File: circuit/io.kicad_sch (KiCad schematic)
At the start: 16 parts, among them J1 Micro_SD_Card, J2 Conn_01x22, J2 VGA, J9 SWD programmer, SW1 Reset, U1 Pico, U10 TXB0104D, U4 TXS0108EPW, U7 74LS393

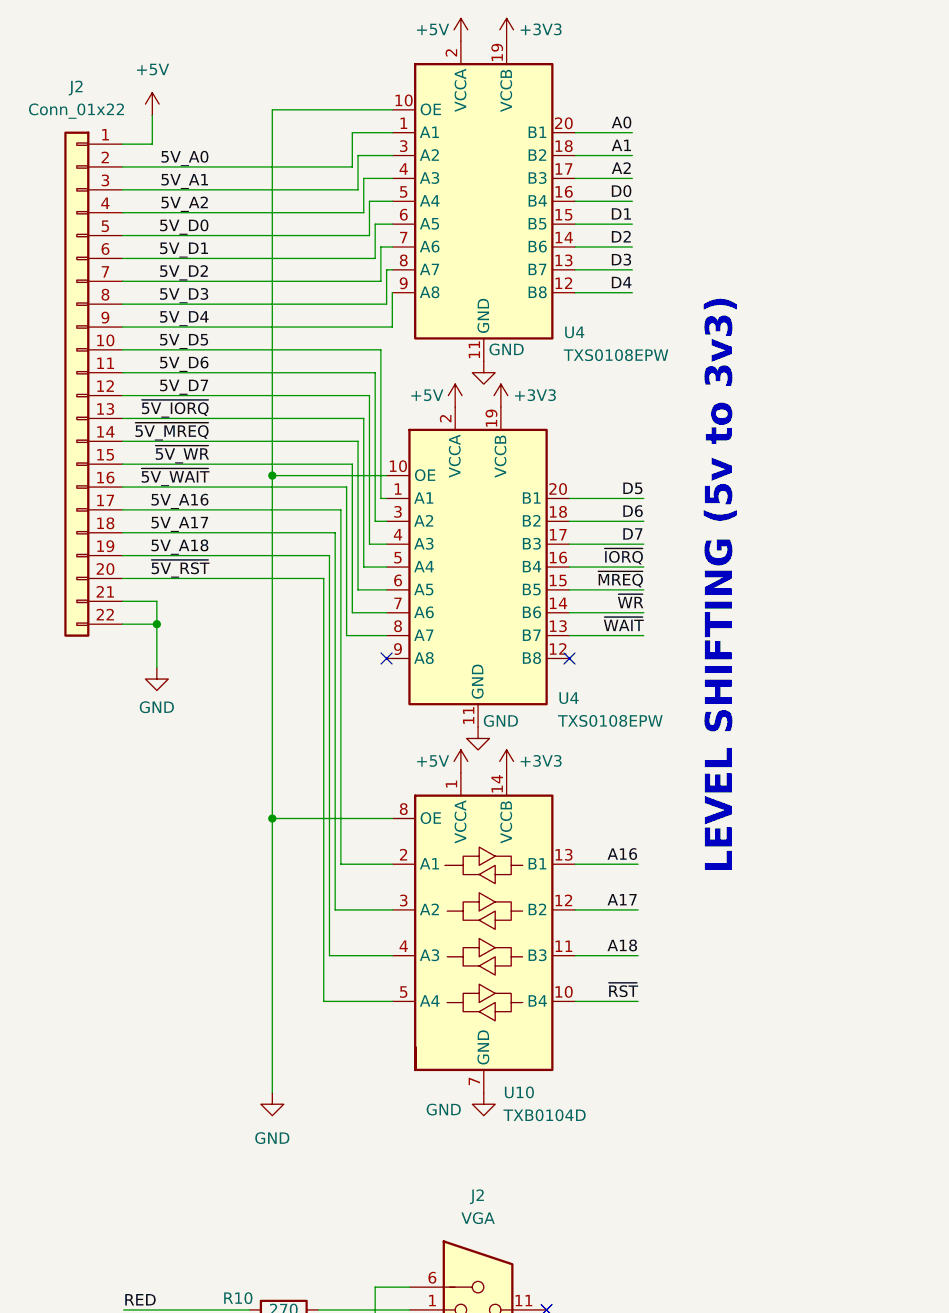
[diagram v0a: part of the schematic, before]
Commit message: .
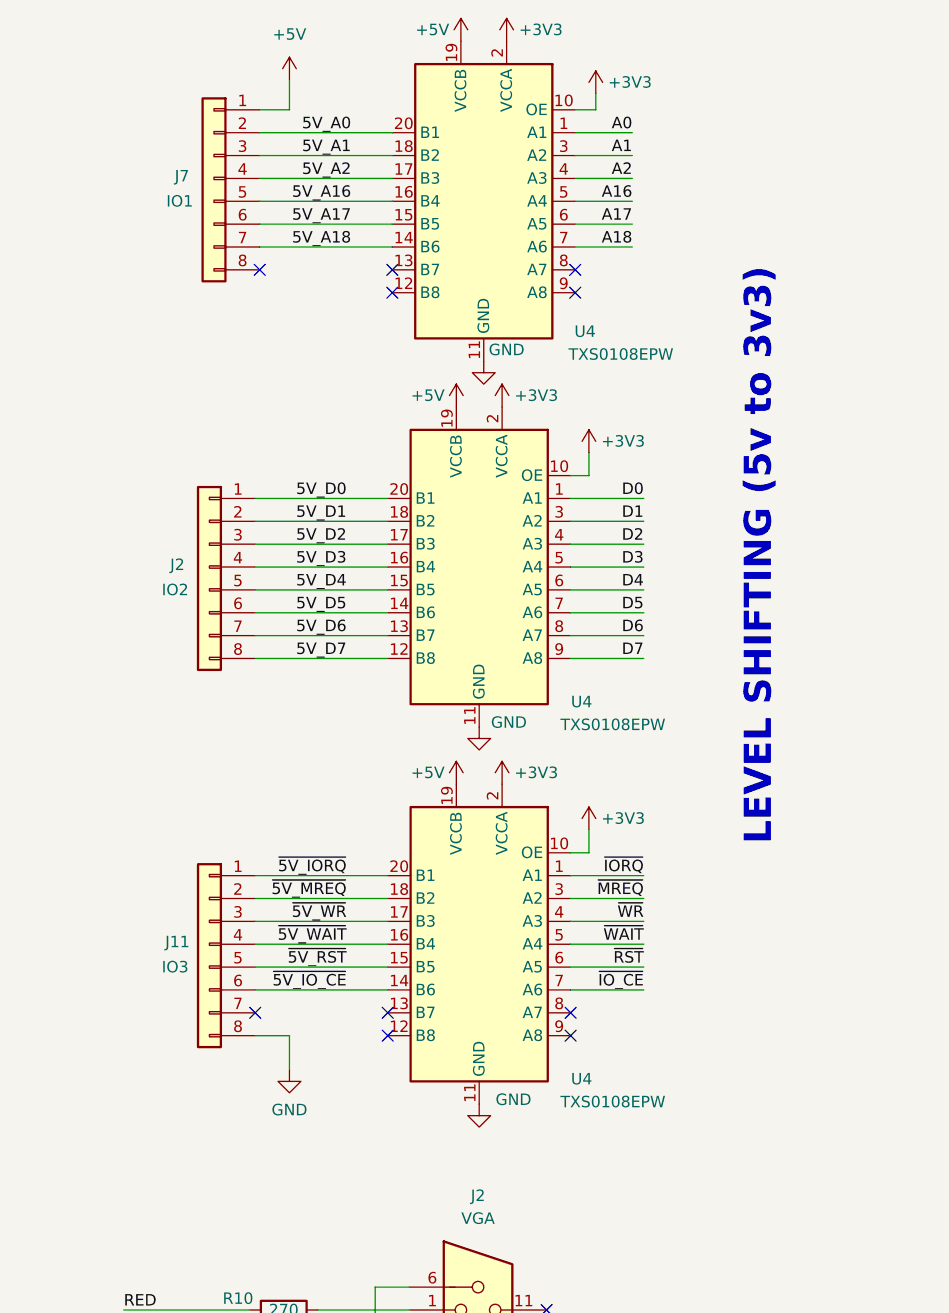
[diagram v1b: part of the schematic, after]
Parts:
- removed J2: Conn_01x22, symbol Connector_Generic:Conn_01x22
- removed U10: TXB0104D, Package_SO:SOIC-14_3.9x8.7mm_P1.27mm, symbol Logic_LevelTranslator:TXB0104D
- added J11: IO3, symbol Connector_Generic:Conn_01x08
- added J2: IO2, symbol Connector_Generic:Conn_01x08
- added J7: IO1, symbol Connector_Generic:Conn_01x08
- added U4: TXS0108EPW, Package_SO:TSSOP-20_4.4x6.5mm_P0.65mm, symbol Logic_LevelTranslator:TXS0108EPW
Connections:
- net +3V3: now also U4.10 (OE), U4.10 (OE), U4.2 (VCCA), U4.2 (VCCA), U4.10 (OE), U4.2 (VCCA); no longer U4.19 (VCCB), U4.19 (VCCB)
- net +5V: now also U4.19 (VCCB), U4.19 (VCCB), J7.1 (Pin_1), U4.19 (VCCB); no longer U4.2 (VCCA), U4.2 (VCCA)
- net 5V_A0: now also U4.20 (B1), J7.2 (Pin_2); no longer U4.1 (A1)
- net 5V_A1: now also U4.18 (B2), J7.3 (Pin_3); no longer U4.3 (A2)
- net 5V_A16: now also U4.16 (B4), J7.5 (Pin_5)
- net 5V_A17: now also U4.15 (B5), J7.6 (Pin_6)
- net 5V_A18: now also U4.14 (B6), J7.7 (Pin_7)
- net 5V_A2: now also U4.17 (B3), J7.4 (Pin_4); no longer U4.4 (A3)
- net 5V_D0: now also U4.20 (B1), J2.1 (Pin_1); no longer U4.5 (A4)
- net 5V_D1: now also U4.18 (B2), J2.2 (Pin_2); no longer U4.6 (A5)
- net 5V_D2: now also U4.17 (B3), J2.3 (Pin_3); no longer U4.7 (A6)
- net 5V_D3: now also U4.16 (B4), J2.4 (Pin_4); no longer U4.8 (A7)
- net 5V_D4: now also U4.15 (B5), J2.5 (Pin_5); no longer U4.9 (A8)
- net 5V_D5: now also U4.14 (B6), J2.6 (Pin_6); no longer U4.1 (A1)
- net 5V_D6: now also U4.13 (B7), J2.7 (Pin_7); no longer U4.3 (A2)
- net 5V_D7: now also U4.12 (B8), J2.8 (Pin_8); no longer U4.4 (A3)
- net A0: now also U4.1 (A1); no longer U4.20 (B1)
- net A1: now also U4.3 (A2); no longer U4.18 (B2)
- net A16: now also U4.5 (A4)
- net A17: now also U4.6 (A5)
- net A18: now also U4.7 (A6)
- net A2: now also U4.4 (A3); no longer U4.17 (B3)
- net D0: now also U4.1 (A1); no longer U4.16 (B4)
- net D1: now also U4.3 (A2); no longer U4.15 (B5)
- net D2: now also U4.4 (A3); no longer U4.14 (B6)
- net D3: now also U4.5 (A4); no longer U4.13 (B7)
- net D4: now also U4.6 (A5); no longer U4.12 (B8)
- net D5: now also U4.7 (A6); no longer U4.20 (B1)
- net D6: now also U4.8 (A7); no longer U4.18 (B2)
- net D7: now also U4.9 (A8); no longer U4.17 (B3)
- net GND: now also J11.8 (Pin_8), U4.11 (GND); no longer U4.10 (OE), U4.10 (OE)
- net ~{5V_IORQ}: now also J11.1 (Pin_1), U4.20 (B1); no longer U4.5 (A4)
- net ~{5V_MREQ}: now also J11.2 (Pin_2), U4.18 (B2); no longer U4.6 (A5)
- net ~{5V_RST}: now also J11.5 (Pin_5), U4.15 (B5)
- net ~{5V_WAIT}: now also J11.4 (Pin_4), U4.16 (B4); no longer U4.8 (A7)
- net ~{5V_WR}: now also J11.3 (Pin_3), U4.17 (B3); no longer U4.7 (A6)
- net ~{IORQ}: now also U4.1 (A1); no longer U4.16 (B4)
- net ~{MREQ}: now also U4.3 (A2); no longer U4.15 (B5)
- net ~{RST}: now also U4.6 (A5)
- net ~{WAIT}: now also U4.5 (A4); no longer U4.13 (B7)
- net ~{WR}: now also U4.4 (A3); no longer U4.14 (B6)
- new net ~{5V_IO_CE}: J11.6 (Pin_6), U4.14 (B6)
- new net ~{IO_CE}: U4.7 (A6)
- no-connect marks 25 -> 33
